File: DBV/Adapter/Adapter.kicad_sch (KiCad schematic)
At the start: 9 parts, among them J1 USB_B, U1 MC68000FN, U2 STM32C071CBUx, U3 AMS1117-3.3

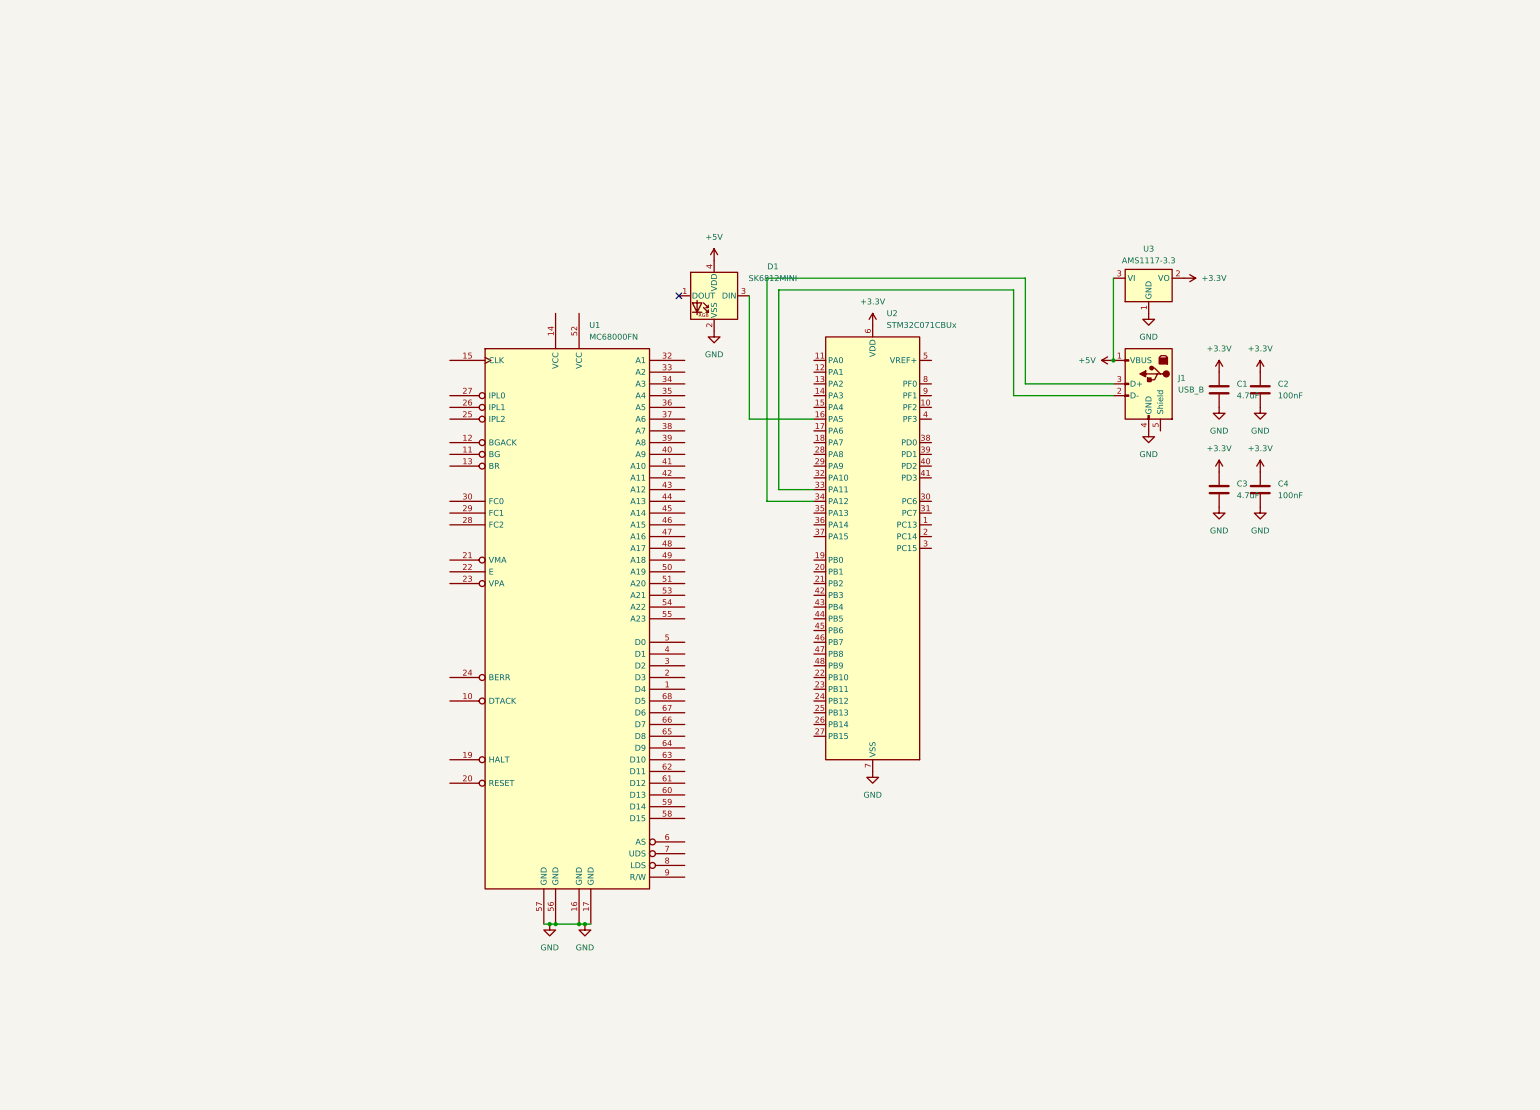
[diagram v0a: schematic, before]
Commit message: plcc68
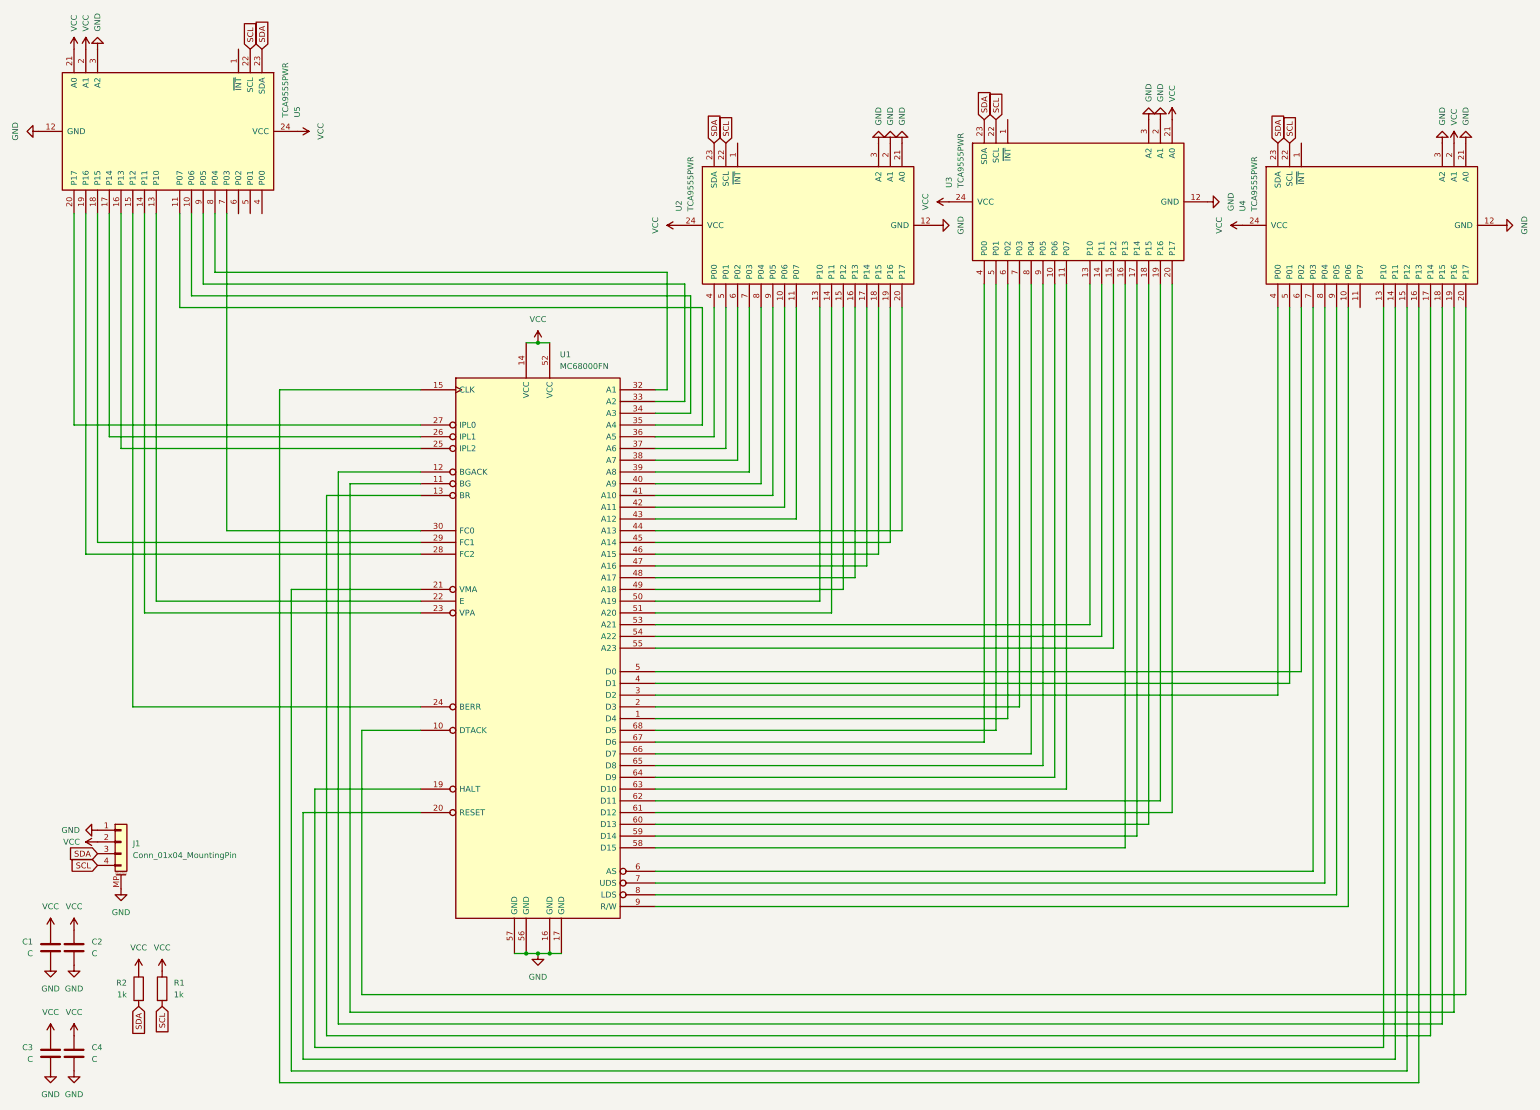
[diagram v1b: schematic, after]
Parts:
- removed D1: SK6812MINI, LED_SMD:LED_SK6812MINI_PLCC4_3.5x3.5mm_P1.75mm, symbol LED:SK6812MINI
- removed J1: USB_B, Connector_USB:USB_B_TE_5787834_Vertical, symbol Connector:USB_B
- removed U2: STM32C071CBUx, Package_DFN_QFN:QFN-48-1EP_7x7mm_P0.5mm_EP5.6x5.6mm, symbol MCU_ST_STM32C0:STM32C071CBUx
- removed U3: AMS1117-3.3, Package_TO_SOT_SMD:SOT-223-3_TabPin2, symbol Regulator_Linear:AMS1117-3.3
- added J1: Conn_01x04_MountingPin, Connector_JST:JST_SH_BM04B-SRSS-TB_1x04-1MP_P1.00mm_Vertical, symbol Connector_Generic_MountingPin:Conn_01x04_MountingPin
- added R1, R2: 1k, Resistor_SMD:R_0603_1608Metric, symbol Device:R
- added U2, U3, U4, U5: TCA9555PWR, Package_SO:TSSOP-24_4.4x7.8mm_P0.65mm, symbol Interface_Expansion:TCA9555PWR
- C1, C3: value 4.7uF -> C; footprint Capacitor_SMD:C_0805_2012Metric -> Capacitor_SMD:C_0603_1608Metric
- C2, C4: value 100nF -> C; footprint Capacitor_SMD:C_0805_2012Metric -> Capacitor_SMD:C_0603_1608Metric
- U1: footprint (none) -> PLCCaussen:PLCC-68_out
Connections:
- net +3.3V is gone; now on net VCC: C1.1, C2.1, C3.1, C4.1
- net GND: now also J1.1 (Pin_1), J1.MP (MountPin), U2.12 (GND), U2.2 (A1), U2.21 (A0), U2.3 (A2), U3.12 (GND), U3.2 (A1), U3.3 (A2), U4.12 (GND), U4.21 (A0), U4.3 (A2), U5.12 (GND), U5.3 (A2)
- net at U1.1 (D4): now also U3.6 (P02)
- net at U1.10 (DTACK): now also U4.20 (P17)
- net at U1.11 (BG): now also U4.19 (P16)
- net at U1.12 (BGACK): now also U4.18 (P15)
- net at U1.13 (BR): now also U4.17 (P14)
- net VCC: now reaches U1.14 (VCC)
- net VCC: now also U1.52 (VCC), J1.2 (Pin_2), R1.1, R2.1, U2.24 (VCC), U3.21 (A0), U3.24 (VCC), U4.2 (A1), U4.24 (VCC), U5.2 (A1), U5.21 (A0), U5.24 (VCC)
- net at U1.15 (CLK): now also U4.16 (P13)
- net at U1.19 (HALT): now also U4.13 (P10)
- net at U1.2 (D3): now also U3.7 (P03)
- net at U1.20 (RESET): now also U4.14 (P11)
- net at U1.21 (VMA): now also U4.15 (P12)
- net at U1.22 (E): now also U5.13 (P10)
- net at U1.23 (VPA): now also U5.14 (P11)
- net at U1.24 (BERR): now also U5.15 (P12)
- net at U1.25 (IPL2): now also U5.16 (P13)
- net at U1.26 (IPL1): now also U5.17 (P14)
- net at U1.27 (IPL0): now also U5.20 (P17)
- net at U1.28 (FC2): now also U5.19 (P16)
- net at U1.29 (FC1): now also U5.18 (P15)
- net at U1.3 (D2): now also U4.4 (P00)
- net at U1.30 (FC0): now also U5.7 (P03)
- net at U1.32 (A1): now also U5.8 (P04)
- net at U1.33 (A2): now also U5.9 (P05)
- net at U1.34 (A3): now also U5.10 (P06)
- net at U1.35 (A4): now also U5.11 (P07)
- net at U1.36 (A5): now also U2.4 (P00)
- net at U1.37 (A6): now also U2.5 (P01)
- net at U1.38 (A7): now also U2.6 (P02)
- net at U1.39 (A8): now also U2.7 (P03)
- net at U1.4 (D1): now also U4.5 (P01)
- net at U1.40 (A9): now also U2.8 (P04)
- net at U1.41 (A10): now also U2.9 (P05)
- net at U1.42 (A11): now also U2.10 (P06)
- net at U1.43 (A12): now also U2.11 (P07)
- net at U1.44 (A13): now also U2.20 (P17)
- net at U1.45 (A14): now also U2.19 (P16)
- net at U1.46 (A15): now also U2.18 (P15)
- net at U1.47 (A16): now also U2.17 (P14)
- net at U1.48 (A17): now also U2.16 (P13)
- net at U1.49 (A18): now also U2.15 (P12)
- net at U1.5 (D0): now also U4.6 (P02)
- net at U1.50 (A19): now also U2.13 (P10)
- net at U1.51 (A20): now also U2.14 (P11)
- net at U1.53 (A21): now also U3.13 (P10)
- net at U1.54 (A22): now also U3.14 (P11)
- net at U1.55 (A23): now also U3.15 (P12)
- net at U1.58 (D15): now also U3.16 (P13)
- net at U1.59 (D14): now also U3.17 (P14)
- net at U1.6 (AS): now also U4.7 (P03)
- net at U1.60 (D13): now also U3.18 (P15)
- net at U1.61 (D12): now also U3.20 (P17)
- net at U1.62 (D11): now also U3.19 (P16)
- net at U1.63 (D10): now also U3.11 (P07)
- net at U1.64 (D9): now also U3.10 (P06)
- net at U1.65 (D8): now also U3.9 (P05)
- net at U1.66 (D7): now also U3.8 (P04)
- net at U1.67 (D6): now also U3.4 (P00)
- net at U1.68 (D5): now also U3.5 (P01)
- net at U1.7 (UDS): now also U4.8 (P04)
- net at U1.8 (LDS): now also U4.9 (P05)
- net at U1.9 (R/W): now also U4.10 (P06)
- new net SCL: J1.4 (Pin_4), R1.2, U2.22 (SCL), U3.22 (SCL), U4.22 (SCL), U5.22 (SCL)
- new net SDA: J1.3 (Pin_3), R2.2, U2.23 (SDA), U3.23 (SDA), U4.23 (SDA), U5.23 (SDA)
- no-connect marks 1 -> 0
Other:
- moved on the sheet: U1
